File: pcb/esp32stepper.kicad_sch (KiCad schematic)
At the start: 88 parts, among them J1 JTAG, J2 Stepper, J3 Display 0.96" 128x96, J4 IO, J5 Qwiic_Vertical, J6 FAN, J7 PWR, J8 USB_C_Receptacle_USB2.0_14P, Q1 IRLML9301, Q2 IRLML9301, SW1 RST, SW2 RotaryEncoder, SW3 BOOT, SW4 B1, SW5 B2, U1 TMC2208-LA, U2 ESP32-S3-MINI-1, U3 MPU-9250, U4 AS5048B, U5 LM555xMM, U6 TPS56339DDC, U7 CH224K, U8 BME280

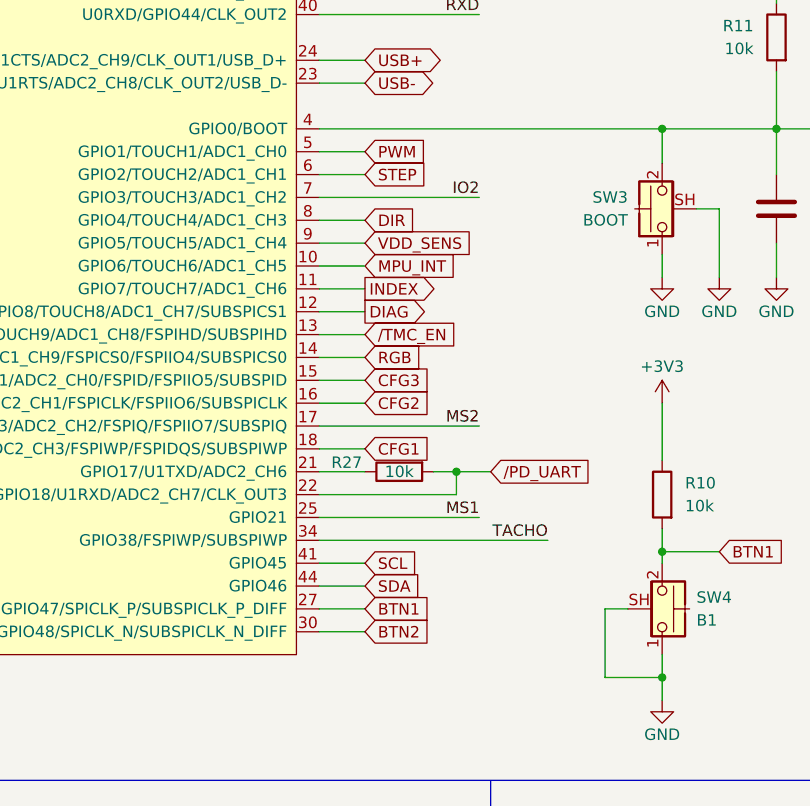
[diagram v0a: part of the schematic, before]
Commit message: update pcb
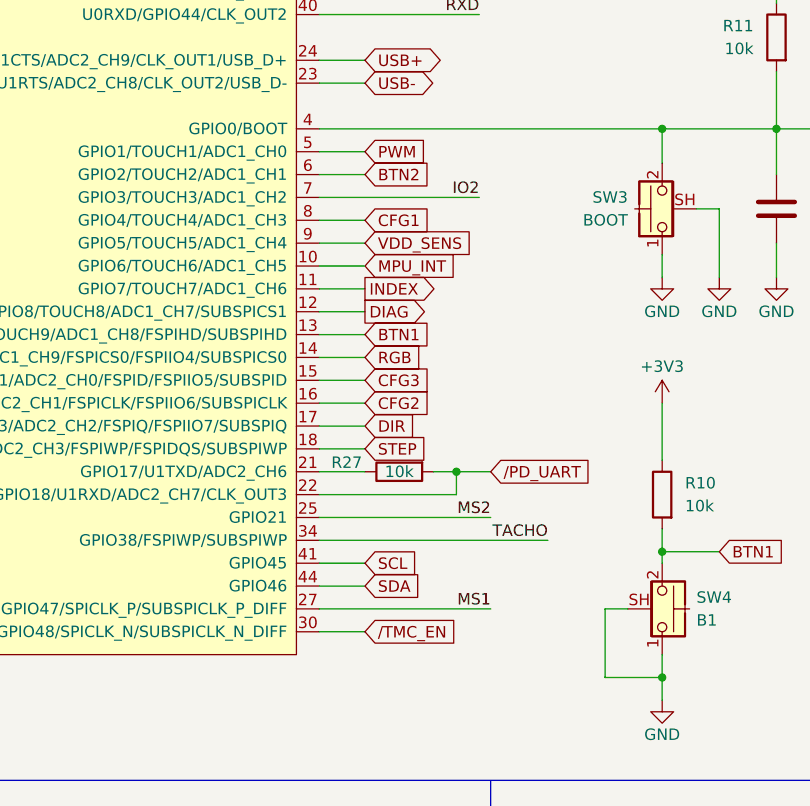
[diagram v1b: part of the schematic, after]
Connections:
- net BTN1: now also U2.13 (GPIO9/TOUCH9/ADC1_CH8/FSPIHD/SUBSPIHD); no longer U2.27 (GPIO47/SPICLK_P/SUBSPICLK_P_DIFF)
- net BTN2: now also U2.6 (GPIO2/TOUCH2/ADC1_CH1); no longer U2.30 (GPIO48/SPICLK_N/SUBSPICLK_N_DIFF)
- net CFG1: now also U2.8 (GPIO4/TOUCH4/ADC1_CH3); no longer U2.18 (GPIO14/TOUCH14/ADC2_CH3/FSPIWP/FSPIDQS/SUBSPIWP)
- net DIR: now also U2.17 (GPIO13/TOUCH13/ADC2_CH2/FSPIQ/FSPIIO7/SUBSPIQ); no longer U2.8 (GPIO4/TOUCH4/ADC1_CH3)
- net MS1: now also U2.27 (GPIO47/SPICLK_P/SUBSPICLK_P_DIFF); no longer U2.25 (GPIO21)
- net MS2: now also U2.25 (GPIO21); no longer U2.17 (GPIO13/TOUCH13/ADC2_CH2/FSPIQ/FSPIIO7/SUBSPIQ)
- net STEP: now also U2.18 (GPIO14/TOUCH14/ADC2_CH3/FSPIWP/FSPIDQS/SUBSPIWP); no longer U2.6 (GPIO2/TOUCH2/ADC1_CH1)
- net /TMC_EN: now also U2.30 (GPIO48/SPICLK_N/SUBSPICLK_N_DIFF); no longer U2.13 (GPIO9/TOUCH9/ADC1_CH8/FSPIHD/SUBSPIHD)
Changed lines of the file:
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@@
 	(wire
 		(pts
-			(xy 165.1 106.68) (xy 182.88 106.68)
+			(xy 165.1 106.68) (xy 170.18 106.68)
 		)
 		(stroke
@@
 	(wire
 		(pts
-			(xy 165.1 116.84) (xy 182.88 116.84)
+			(xy 165.1 116.84) (xy 184.15 116.84)
 		)
 		(stroke
@@
 	(wire
 		(pts
-			(xy 170.18 127) (xy 165.1 127)
+			(xy 184.15 127) (xy 165.1 127)
 		)
 		(stroke
@@
 	)
 	(label "MS2"
-		(at 182.88 106.68 180)
+		(at 184.15 116.84 180)
 		(effects
 			(font
@@
 	)
 	(label "MS1"
-		(at 182.88 116.84 180)
+		(at 184.15 127 180)
 		(effects
 			(font
@@
 	(global_label "BTN2"
 		(shape input)
-		(at 170.18 129.54 0)
+		(at 170.18 78.74 0)
 		(fields_autoplaced yes)
 		(effects
@@
 		)
 		(property "Intersheetrefs" "${INTERSHEET_REFS}"
-			(at 177.9428 129.54 0)
+			(at 177.9428 78.74 0)
 			(effects
 				(font
@@
 	(global_label "BTN1"
 		(shape input)
-		(at 170.18 127 0)
+		(at 170.18 96.52 0)
 		(fields_autoplaced yes)
 		(effects
@@
 		)
 		(property "Intersheetrefs" "${INTERSHEET_REFS}"
-			(at 177.9428 127 0)
+			(at 177.9428 96.52 0)
 			(effects
 				(font
@@
 	(global_label "{slash}TMC_EN"
 		(shape input)
-		(at 170.18 96.52 0)
+		(at 170.18 129.54 0)
 		(fields_autoplaced yes)
 		(effects
@@
 		)
 		(property "Intersheetrefs" "${INTERSHEET_REFS}"
-			(at 181.6318 96.52 0)
+			(at 181.6318 129.54 0)
 			(effects
 				(font
@@
 	(global_label "DIR"
 		(shape input)
-		(at 170.18 83.82 0)
+		(at 170.18 106.68 0)
 		(fields_autoplaced yes)
 		(effects
@@
 		)
 		(property "Intersheetrefs" "${INTERSHEET_REFS}"
-			(at 176.31 83.82 0)
+			(at 176.31 106.68 0)
 			(effects
 				(font
@@
 	(global_label "CFG1"
 		(shape input)
-		(at 170.18 109.22 0)
+		(at 170.18 83.82 0)
 		(fields_autoplaced yes)
 		(effects
@@
 		)
 		(property "Intersheetrefs" "${INTERSHEET_REFS}"
-			(at 178.0033 109.22 0)
+			(at 178.0033 83.82 0)
 			(effects
 				(font
@@
 	(global_label "STEP"
 		(shape input)
-		(at 170.18 78.74 0)
+		(at 170.18 109.22 0)
 		(fields_autoplaced yes)
 		(effects
@@
 		)
 		(property "Intersheetrefs" "${INTERSHEET_REFS}"
-			(at 177.7613 78.74 0)
+			(at 177.7613 109.22 0)
 			(effects
 				(font
